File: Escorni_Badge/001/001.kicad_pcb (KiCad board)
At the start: 2 copper layers, 94.7 x 92.7 mm, 2 parts

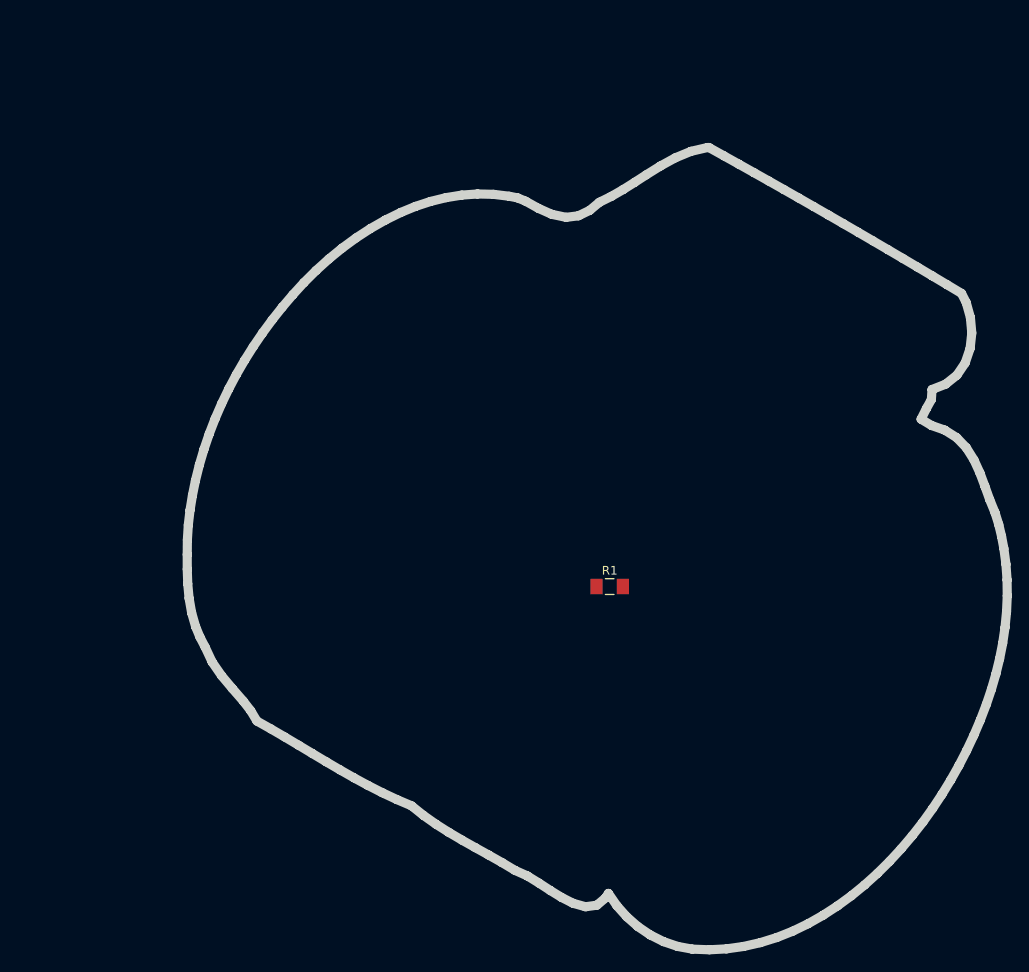
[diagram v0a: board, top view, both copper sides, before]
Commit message: Update Escorni
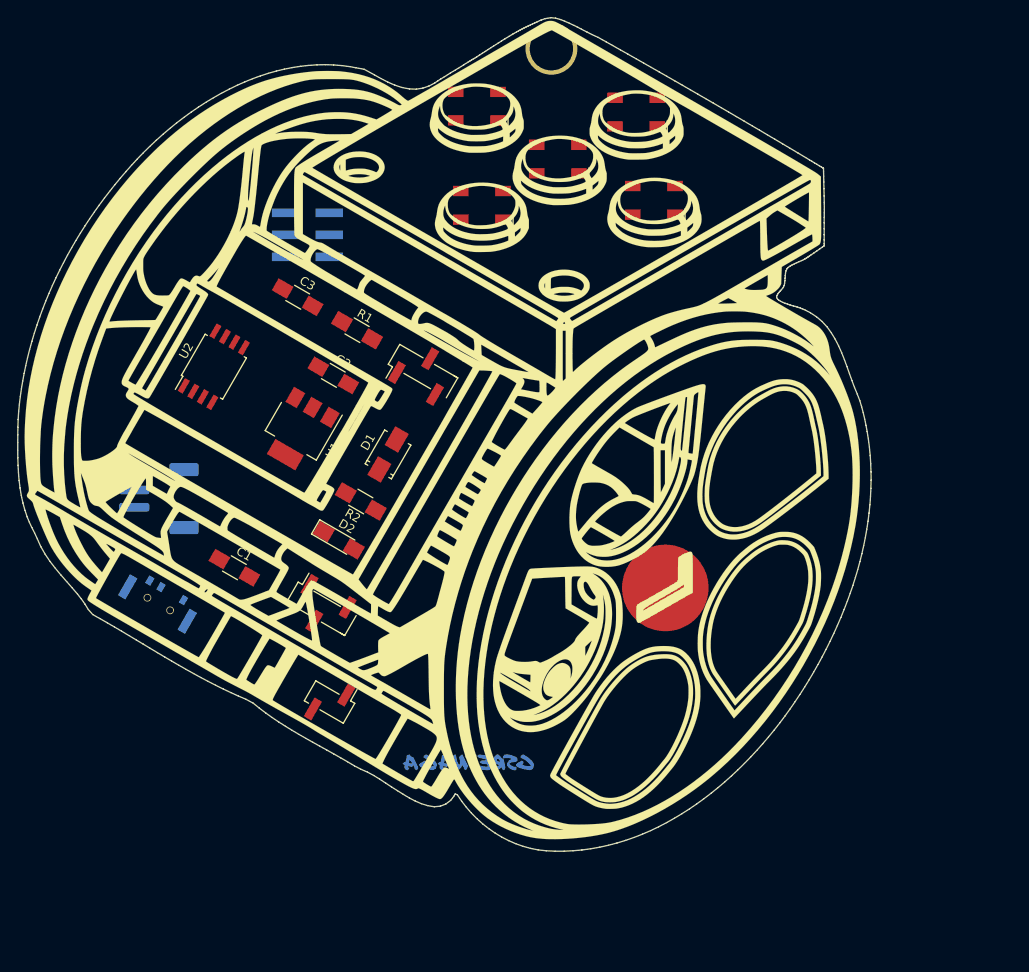
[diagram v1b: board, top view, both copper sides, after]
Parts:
- removed the svg2mod at (146.7, 101.6)
- added C1: 4.7uF, 001:C_1206_HandSoldering, F.Cu at (105.9, 105.1)
- added C2: 4.7uF, 001:C_1206_HandSoldering, F.Cu at (117.3, 82.9)
- added C3: 22nF, 001:C_1206_HandSoldering, F.Cu at (113.2, 73.9)
- added CAP1: Escorni_Touch, 001:escorni-Touch_02_100mm, F.Cu at (155.7, 107.5)
- added D1: MBRA140, 001:DIODE-SMA, F.Cu at (123.6, 92.0)
- added D2: ON, 001:LED_1206_HandSoldering, F.Cu at (117.9, 102.0)
- added J1: CONN_01X02, 001:Pin_Header_Straight_1x02_Pitch2.54mm_SMD_Pin1Left, F.Cu at (116.9, 120.7)
- added J2: CONN_01X02, Connector_JST:JST_PH_S2B-PH-SM4-TB_1x02-1MP_P2.00mm_Horizontal, B.Cu at (97.2, 97.2)
- added J3: CONN_02X03, 001:Pin_Header_Straight_2x03_Pitch2.54mm_SMD, B.Cu at (114.3, 66.7)
- added J4: CONN_01X03, 001:Pin_Header_Straight_1x03_Pitch2.54mm_SMD_Pin1Left, F.Cu at (127.7, 82.4)
- added J5: CONN_01X03, 001:Pin_Header_Straight_1x03_Pitch2.54mm_SMD_Pin1Right, F.Cu at (115.9, 109.9)
- added LED1: WS2812B, 001:WS2812B, F.Cu at (134.5, 63.3)
- added LED2: WS2812B, 001:WS2812B, F.Cu at (154.3, 62.7)
- added LED3: WS2812B, 001:WS2812B, F.Cu at (152.3, 52.5)
- added LED4: WS2812B, 001:WS2812B, F.Cu at (133.9, 51.8)
- added LED5: WS2812B, 001:WS2812B, F.Cu at (143.2, 57.9)
- added MountinHoleBagde: MountingHole_5mm_Badge, 001:MountingHole_3.5mm_Pad, F.Cu at (142.5, 45.2)
- added R2: 1k, 001:R_1206_HandSoldering, F.Cu at (120.5, 97.5)
- added REF**: KiCad-Logo2_6mm_SilkScreen, 001:KiCad-Logo2_6mm_SilkScreen, B.Cu at (156.5, 81.7)
- added S1: MSK12C02_SWITCH-SLIDE-SPDT, 001:MSK12C02, B.Cu at (99.7, 112.4)
- added SilKs1: Escorni_Art, 001:escorni-badge-new_02_100mm, F.Cu at (130.2, 89.4)
- added U1: LM340MP-5.0/NOPB, Package_TO_SOT_SMD:SOT-223-3_TabPin2, F.Cu at (113.3, 89.3)
- added U2: ATTINY85-20SU, Package_SO:SOIJ-8_5.3x5.3mm_P1.27mm, F.Cu at (103.5, 81.9)
- added svg2mod: G***, 001:FirmaCuMask, B.Cu at (132.9, 127.6)
- R1: value R -> 1Mohm; footprint Resistor_SMD:R_1206_3216Metric_Pad1.39x1.80mm_HandSolder -> 001:R_1206_HandSoldering
- moved R1 41.6 mm to (120.0, 77.7), turned to 150 degrees
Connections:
- R1 pad 1: +3.3V -> MISO-1-PWM
- R1 pad 2: GND -> MOSI-0-PWM
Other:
- board size 94.7 x 92.7 mm -> 98.6 x 96.3 mm
- board text added: "Developed by"
